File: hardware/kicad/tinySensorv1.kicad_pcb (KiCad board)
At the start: 2 copper layers, 94 x 60 mm, 31 parts, among them J1 RADIO, J10 CR2032 socket, J11 AAA socket, J12 AA Socket, J13 Bornier, J2 DCDC converter, J3 BMP/BME breakout, J5 OneWire sensor, J6 ISP, J7 Analog sensor, U1 ATtiny84A-PU

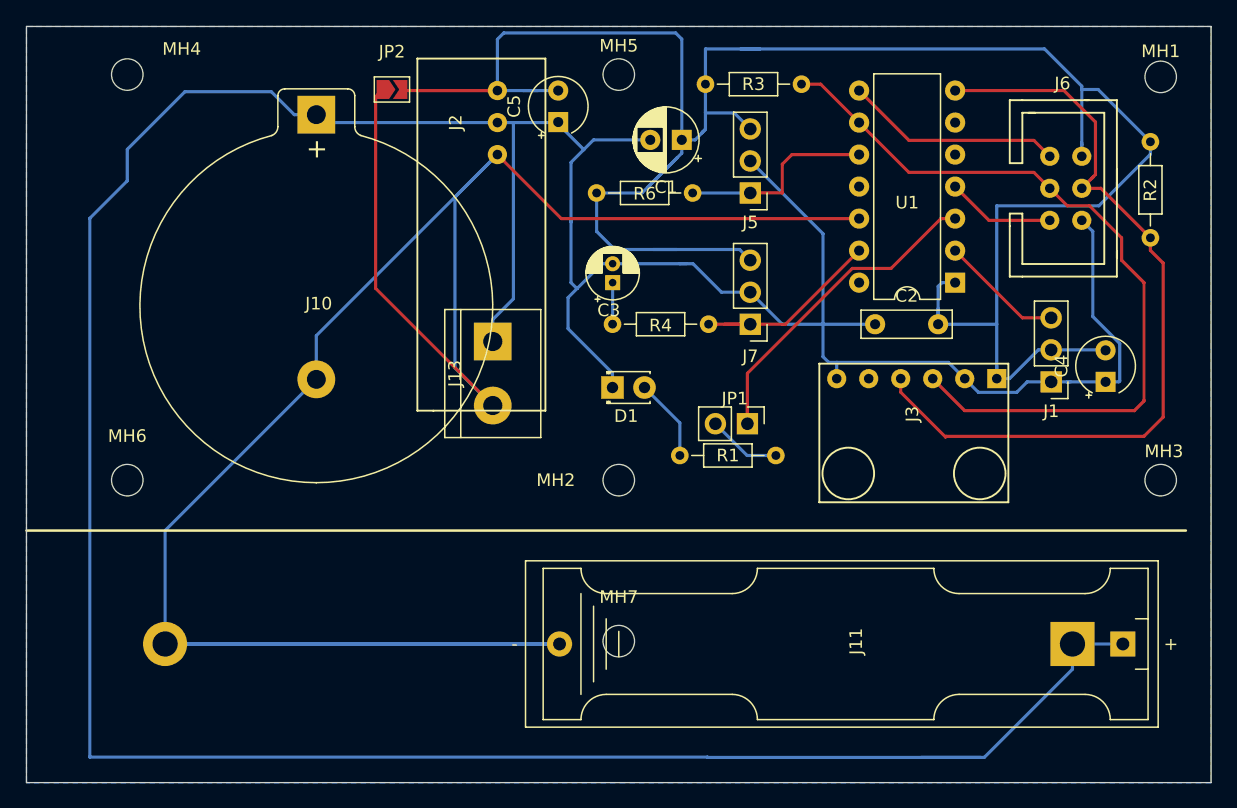
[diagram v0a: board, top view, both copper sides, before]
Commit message: Alpha of pcb version 2
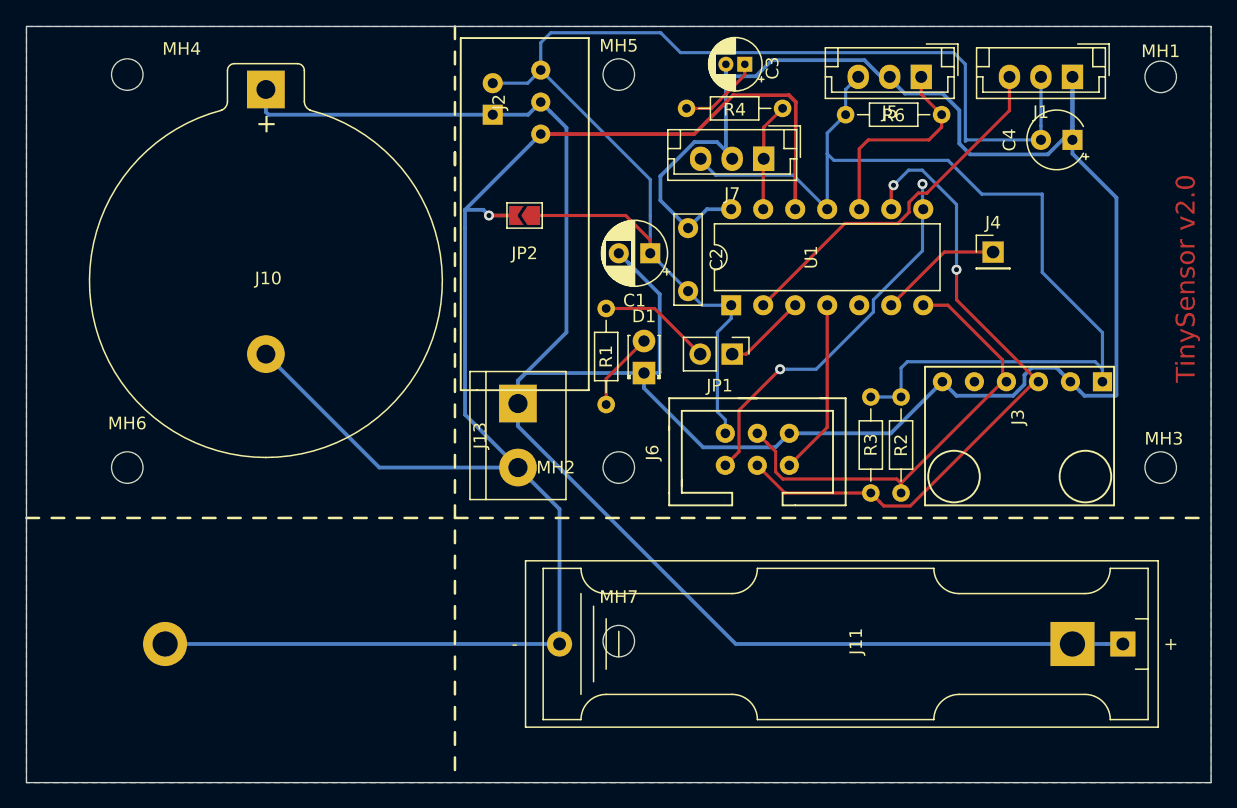
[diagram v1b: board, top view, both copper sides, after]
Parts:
- added J4: PWM_OUT, Connector_PinHeader_2.54mm:PinHeader_1x01_P2.54mm_Vertical, F.Cu at (189.7, 65.9)
- C5: moved to B.Cu
- J1, J5, J7: footprint Connector_PinHeader_2.54mm:PinHeader_1x03_P2.54mm_Vertical -> Connector_JST:JST_EH_B03B-EH-A_1x03_P2.50mm_Vertical
- J13: value Bornier -> RAW IN
- moved J6 41.9 mm to (164.0, 85.0), turned to 0 degrees
- moved R2 28.3 mm to (182.4, 77.4)
- moved R3 28.1 mm to (180.0, 77.4), turned to 270 degrees
- moved J1 24.3 mm to (196.0, 52.0)
- moved R6 20.7 mm to (178.0, 55.0)
- moved C3 20.3 mm to (170.0, 51.0), turned to 180 degrees
- moved C4 19.4 mm to (196.0, 57.0), turned to 180 degrees
- moved R4 18.1 mm to (173.0, 54.5)
- moved U1 17.9 mm to (168.9, 70.1), turned to 90 degrees
- moved C2 16.7 mm to (165.5, 64.0), turned to 270 degrees
- moved J5 16.4 mm to (184.0, 52.0)
- moved JP2 14.5 mm to (152.5, 63.0), turned to 180 degrees
- moved J7 13.2 mm to (171.5, 58.5)
- moved C1 9.34 mm to (162.5, 66.0)
- moved J3 8.39 mm to (193.3, 80.0)
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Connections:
- C1 pad 1: +3V3 -> VCC
- C2 pad 2: +3V3 -> VCC
- C4 pad 2: +3V3 -> VCC
- C5 pad 2: +3V3 -> VCC
- J1 pad 2: +3V3 -> VCC
- J2 pad 3: +3V3 -> VCC
- J3 pad 1: +3V3 -> /SENSOR_VCC
- J5 pad 3: +3V3 -> /SENSOR_VCC
- J6 pad 2: +3V3 -> VCC
- J7 pad 3: +3V3 -> /SENSOR_VCC
- JP2 pad 1: +BATT -> VCC
- JP2 pad 2: +3V3 -> +BATT
- R2 pad 1: +3V3 -> /SENSOR_VCC
- R3 pad 1: +3V3 -> /SENSOR_VCC
- R6 pad 1: +3V3 -> /SENSOR_VCC
- U1 pad 1: +3V3 -> VCC
- U1 pad 11: Net-(U1-Pad11) -> /SENSOR_VCC
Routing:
- net +3V3: track 185.8 -> 0.00 mm
- net VCC: track 0.00 -> 106.9 mm
- net /SENSOR_VCC: track 0.00 -> 80.7 mm
- net +BATT: track 194.2 -> 135.5 mm, vias 0 -> 1
- net GND: track 311.9 -> 266.0 mm
- net /SDA: track 63.8 -> 36.0 mm
- net /LED_OUT: track 27.3 -> 6.61 mm
- net /TX_RADIO: track 9.83 -> 29.1 mm
- net /MISO: track 17.3 -> 30.5 mm, vias 0 -> 2
- net /PWM_OUT: track 0.00 -> 9.83 mm
- net /SCL: track 62.3 -> 52.8 mm, vias 0 -> 2
- net /Analog_sensor: track 16.4 -> 8.64 mm
- net /RESET: track 8.62 -> 14.0 mm
- net Net-(C3-Pad1): track 3.30 -> 6.57 mm
- net Net-(JP1-Pad2): track 5.84 -> 8.96 mm
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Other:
- net class power added: clearance 0.2, trace_width 0.3, via_dia 0.8, via_drill 0.4
- board text added: "TinySensor v2.0"
